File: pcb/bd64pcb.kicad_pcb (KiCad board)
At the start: 2 copper layers, 266.7 x 95.2 mm, 226 parts, among them J1 USB_C_Receptacle_USB2.0, SW1 SW_Push, U1 ATmega32U4-MU, U3 IS31FL3733-QF, Y1 16MHz

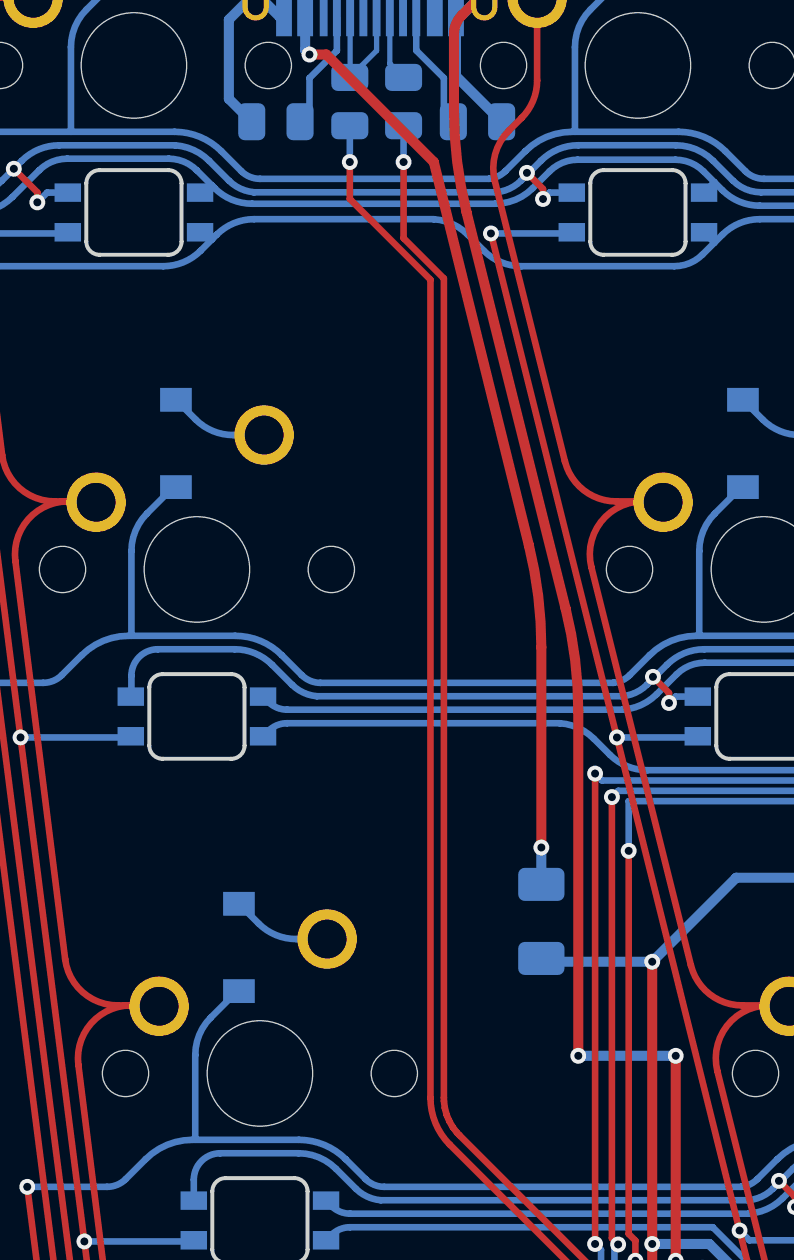
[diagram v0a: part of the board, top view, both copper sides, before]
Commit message: fillet touchups
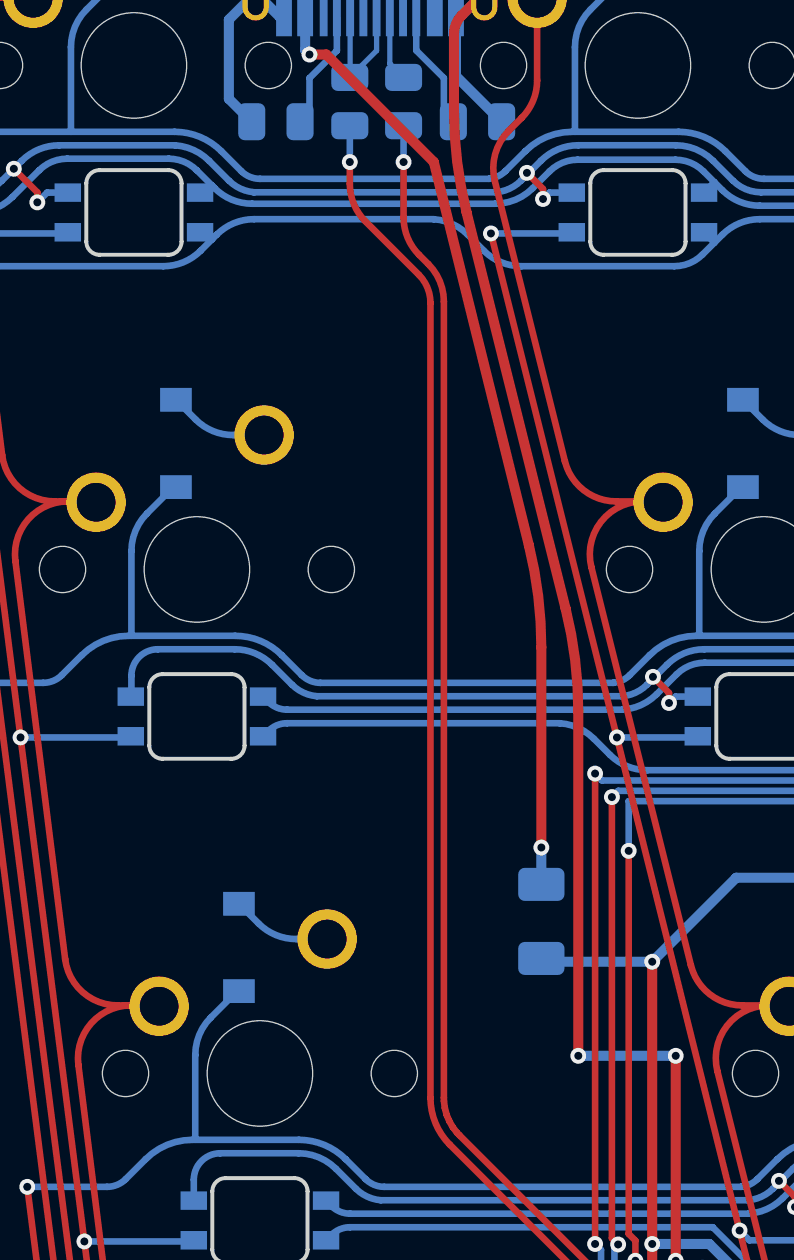
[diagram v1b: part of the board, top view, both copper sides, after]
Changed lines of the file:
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@@
   (segment (start 40.288292 102.967708) (end 41.211281 102.967708) (width 0.25) (layer "B.Cu") (net 121))
   (segment (start 30.535 99.369) (end 26.976 99.369) (width 0.25) (layer "B.Cu") (net 121))
-  (segment (start 34.798 55.245) (end 34.798 58.123136) (width 0.25) (layer "F.Cu") (net 122))
-  (segment (start 36.323927 90.742534) (end 36.358112 91.002216) (width 0.25) (layer "F.Cu") (net 122))
-  (segment (start 44.15085 99.861232) (end 44.193581 100.185833) (width 0.25) (layer "F.Cu") (net 122))
-  (segment (start 36.907787 92.025787) (end 43.463767 98.581767) (width 0.25) (layer "F.Cu") (net 122))
-  (segment (start 36.52613 91.497201) (end 36.657089 91.724033) (width 0.25) (layer "F.Cu") (net 122))
-  (segment (start 44.196 100.349534) (end 44.196 110.617) (width 0.25) (layer "F.Cu") (net 122))
-  (segment (start 43.463767 98.581767) (end 43.577824 98.699217) (width 0.25) (layer "F.Cu") (net 122))
-  (segment (start 34.798 58.123136) (end 36.322 59.647136) (width 0.25) (layer "F.Cu") (net 122))
   (segment (start 36.358112 91.002216) (end 36.425899 91.255215) (width 0.25) (layer "F.Cu") (net 122))
   (segment (start 36.816535 91.931832) (end 36.907787 92.025787) (width 0.25) (layer "F.Cu") (net 122))
+  (segment (start 44.066117 99.544985) (end 44.15085 99.861232) (width 0.25) (layer "F.Cu") (net 122))
+  (segment (start 36.52613 91.497201) (end 36.657089 91.724033) (width 0.25) (layer "F.Cu") (net 122))
+  (segment (start 36.907787 92.025787) (end 43.463767 98.581767) (width 0.25) (layer "F.Cu") (net 122))
+  (segment (start 36.322 60.518427) (end 36.322 90.611573) (width 0.25) (layer "F.Cu") (net 122))
+  (segment (start 44.193581 100.185833) (end 44.196 100.349534) (width 0.25) (layer "F.Cu") (net 122))
+  (segment (start 43.577824 98.699217) (end 43.777131 98.958965) (width 0.25) (layer "F.Cu") (net 122))
+  (segment (start 34.798 55.245) (end 34.798 57.337573) (width 0.25) (layer "F.Cu") (net 122))
+  (segment (start 43.463767 98.581767) (end 43.577824 98.699217) (width 0.25) (layer "F.Cu") (net 122))
+  (segment (start 44.15085 99.861232) (end 44.193581 100.185833) (width 0.25) (layer "F.Cu") (net 122))
+  (segment (start 43.940829 99.242504) (end 44.066117 99.544985) (width 0.25) (layer "F.Cu") (net 122))
   (segment (start 36.425899 91.255215) (end 36.52613 91.497201) (width 0.25) (layer "F.Cu") (net 122))
-  (segment (start 43.577824 98.699217) (end 43.777131 98.958965) (width 0.25) (layer "F.Cu") (net 122))
-  (segment (start 36.322 59.647136) (end 36.322 90.611573) (width 0.25) (layer "F.Cu") (net 122))
-  (segment (start 44.066117 99.544985) (end 44.15085 99.861232) (width 0.25) (layer "F.Cu") (net 122))
+  (segment (start 44.196 100.349534) (end 44.196 110.617) (width 0.25) (layer "F.Cu") (net 122))
+  (segment (start 35.383787 58.751787) (end 35.736214 59.104214) (width 0.25) (layer "F.Cu") (net 122))
+  (segment (start 36.322 90.611573) (end 36.323927 90.742534) (width 0.25) (layer "F.Cu") (net 122))
   (segment (start 36.657089 91.724033) (end 36.816535 91.931832) (width 0.25) (layer "F.Cu") (net 122))
-  (segment (start 36.322 90.611573) (end 36.323927 90.742534) (width 0.25) (layer "F.Cu") (net 122))
-  (segment (start 44.193581 100.185833) (end 44.196 100.349534) (width 0.25) (layer "F.Cu") (net 122))
-  (segment (start 43.940829 99.242504) (end 44.066117 99.544985) (width 0.25) (layer "F.Cu") (net 122))
   (segment (start 43.777131 98.958965) (end 43.940829 99.242504) (width 0.25) (layer "F.Cu") (net 122))
+  (segment (start 36.323927 90.742534) (end 36.358112 91.002216) (width 0.25) (layer "F.Cu") (net 122))
   (via (at 44.196 110.617) (size 0.6) (drill 0.3) (layers "F.Cu" "B.Cu") (net 122))
   (via (at 34.798 55.245) (size 0.6) (drill 0.3) (layers "F.Cu" "B.Cu") (net 122))
+  (arc (start 34.798 57.337573) (mid 34.950241 58.10294) (end 35.383787 58.751787) (width 0.25) (layer "F.Cu") (net 122))
+  (arc (start 36.322 60.518427) (mid 36.169759 59.75306) (end 35.736214 59.104214) (width 0.25) (layer "F.Cu") (net 122))
   (segment (start 42.996489 108.023725) (end 43.686138 107.334076) (width 0.25) (layer "B.Cu") (net 122))
   (segment (start 42.996489 110.117) (end 42.996489 108.023725) (width 0.25) (layer "B.Cu") (net 122))
@@
   (segment (start 42.29952 78.62152) (end 156.83648 78.62152) (width 0.25) (layer "B.Cu") (net 125))
   (segment (start 153.924 45.085) (end 152.781 46.228) (width 0.25) (layer "B.Cu") (net 125))
-  (segment (start 32.766 55.245) (end 32.766 56.642) (width 0.25) (layer "F.Cu") (net 126))
-  (segment (start 43.688 109.855) (end 43.561 109.982) (width 0.25) (layer "F.Cu") (net 126))
-  (segment (start 32.766 56.642) (end 35.814 59.69) (width 0.25) (layer "F.Cu") (net 126))
-  (segment (start 35.814 59.69) (end 35.814 90.616398) (width 0.25) (layer "F.Cu") (net 126))
+  (segment (start 33.351787 57.481787) (end 35.37466 59.50466) (width 0.25) (layer "F.Cu") (net 126))
   (segment (start 36.546233 92.384165) (end 43.102214 98.940146) (width 0.25) (layer "F.Cu") (net 126))
   (segment (start 43.688 100.354359) (end 43.688 109.855) (width 0.25) (layer "F.Cu") (net 126))
+  (segment (start 35.814 60.56532) (end 35.814 90.616398) (width 0.25) (layer "F.Cu") (net 126))
+  (segment (start 43.688 109.855) (end 43.561 109.982) (width 0.25) (layer "F.Cu") (net 126))
+  (segment (start 32.766 55.245) (end 32.766 56.067573) (width 0.25) (layer "F.Cu") (net 126))
   (via (at 32.766 55.245) (size 0.6) (drill 0.3) (layers "F.Cu" "B.Cu") (net 126))
   (via (at 43.561 109.982) (size 0.6) (drill 0.3) (layers "F.Cu" "B.Cu") (net 126))
+  (arc (start 32.766 56.067573) (mid 32.918241 56.83294) (end 33.351787 57.481787) (width 0.25) (layer "F.Cu") (net 126))
+  (arc (start 35.814 90.616398) (mid 36.004301 91.573107) (end 36.546233 92.384165) (width 0.25) (layer "F.Cu") (net 126))
   (arc (start 43.102214 98.940146) (mid 43.535759 99.588992) (end 43.688 100.354359) (width 0.25) (layer "F.Cu") (net 126))
-  (arc (start 35.814 90.616398) (mid 36.004301 91.573107) (end 36.546233 92.384165) (width 0.25) (layer "F.Cu") (net 126))
+  (arc (start 35.37466 59.50466) (mid 35.699819 59.991295) (end 35.814 60.56532) (width 0.25) (layer "F.Cu") (net 126))
   (segment (start 32.766 55.245) (end 32.766 53.8715) (width 0.25) (layer "B.Cu") (net 126))
   (segment (start 44.039691 107.687629) (end 43.519188 108.208132) (width 0.25) (layer "B.Cu") (net 126))
